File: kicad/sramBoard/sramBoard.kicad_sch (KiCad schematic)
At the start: 1 part, among them J1 Conn_02x20_Top_Bottom

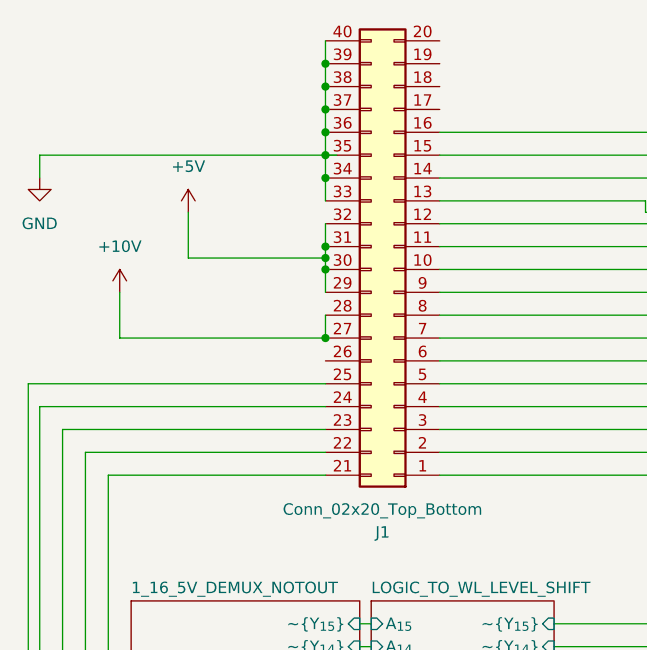
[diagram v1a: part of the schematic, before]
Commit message: cdcdcdcdcdcdcdcdcdcdc
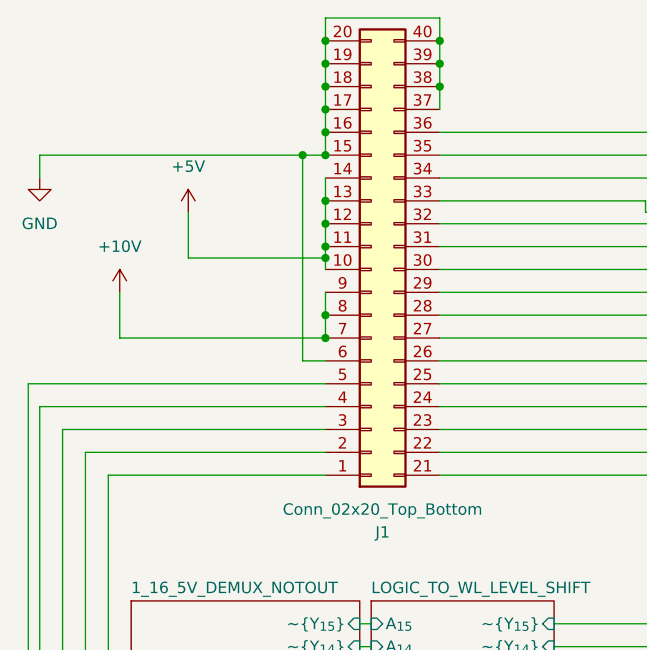
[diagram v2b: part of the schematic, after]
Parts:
- J1: footprint (none) -> Connector_IDC:IDC-Header_2x20_P2.54mm_Horizontal
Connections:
- net +10V: now also J1.7 (Pin_7), J1.8 (Pin_8), J1.9 (Pin_9); no longer J1.27 (Pin_27), J1.28 (Pin_28)
- net +5V: now also J1.10 (Pin_10), J1.11 (Pin_11), J1.12 (Pin_12), J1.13 (Pin_13), J1.14 (Pin_14); no longer J1.29 (Pin_29), J1.30 (Pin_30), J1.31 (Pin_31), J1.32 (Pin_32)
- net 1_16_5V_DEMUX_NOTOUT/D: now also J1.5 (Pin_5); no longer J1.25 (Pin_25)
- net 1_16_5V_DEMUX_NOTOUT/S_{0}: now also J1.1 (Pin_1); no longer J1.21 (Pin_21)
- net 1_16_5V_DEMUX_NOTOUT/S_{1}: now also J1.2 (Pin_2); no longer J1.22 (Pin_22)
- net 1_16_5V_DEMUX_NOTOUT/S_{2}: now also J1.3 (Pin_3); no longer J1.23 (Pin_23)
- net 1_16_5V_DEMUX_NOTOUT/S_{3}: now also J1.4 (Pin_4); no longer J1.24 (Pin_24)
- net 8BIT_ROW15/BL_{0}_: now also J1.21 (Pin_21); no longer J1.1 (Pin_1)
- net 8BIT_ROW15/BL_{1}_: now also J1.23 (Pin_23); no longer J1.3 (Pin_3)
- net 8BIT_ROW15/BL_{2}_: now also J1.25 (Pin_25); no longer J1.5 (Pin_5)
- net 8BIT_ROW15/BL_{3}_: now also J1.27 (Pin_27); no longer J1.7 (Pin_7)
- net 8BIT_ROW15/BL_{4}_: now also J1.29 (Pin_29); no longer J1.9 (Pin_9)
- net 8BIT_ROW15/BL_{5}_: now also J1.31 (Pin_31); no longer J1.11 (Pin_11)
- net 8BIT_ROW15/BL_{6}_: now also J1.33 (Pin_33); no longer J1.13 (Pin_13)
- net 8BIT_ROW15/BL_{7}_: now also J1.35 (Pin_35); no longer J1.15 (Pin_15)
- net 8BIT_ROW15/~{BL_{0}}_: now also J1.22 (Pin_22); no longer J1.2 (Pin_2)
- net 8BIT_ROW15/~{BL_{1}}_: now also J1.24 (Pin_24); no longer J1.4 (Pin_4)
- net 8BIT_ROW15/~{BL_{2}}_: now also J1.26 (Pin_26); no longer J1.6 (Pin_6)
- net 8BIT_ROW15/~{BL_{3}}_: now also J1.28 (Pin_28); no longer J1.8 (Pin_8)
- net 8BIT_ROW15/~{BL_{4}}_: now also J1.30 (Pin_30); no longer J1.10 (Pin_10)
- net 8BIT_ROW15/~{BL_{5}}_: now also J1.32 (Pin_32); no longer J1.12 (Pin_12)
- net 8BIT_ROW15/~{BL_{6}}_: now also J1.34 (Pin_34); no longer J1.14 (Pin_14)
- net 8BIT_ROW15/~{BL_{7}}_: now also J1.36 (Pin_36); no longer J1.16 (Pin_16)
- net GND: now also J1.15 (Pin_15), J1.16 (Pin_16), J1.17 (Pin_17), J1.18 (Pin_18), J1.19 (Pin_19), J1.20 (Pin_20), J1.6 (Pin_6); no longer J1.33 (Pin_33), J1.34 (Pin_34), J1.35 (Pin_35), J1.36 (Pin_36)
